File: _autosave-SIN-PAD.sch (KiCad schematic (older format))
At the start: 12 parts

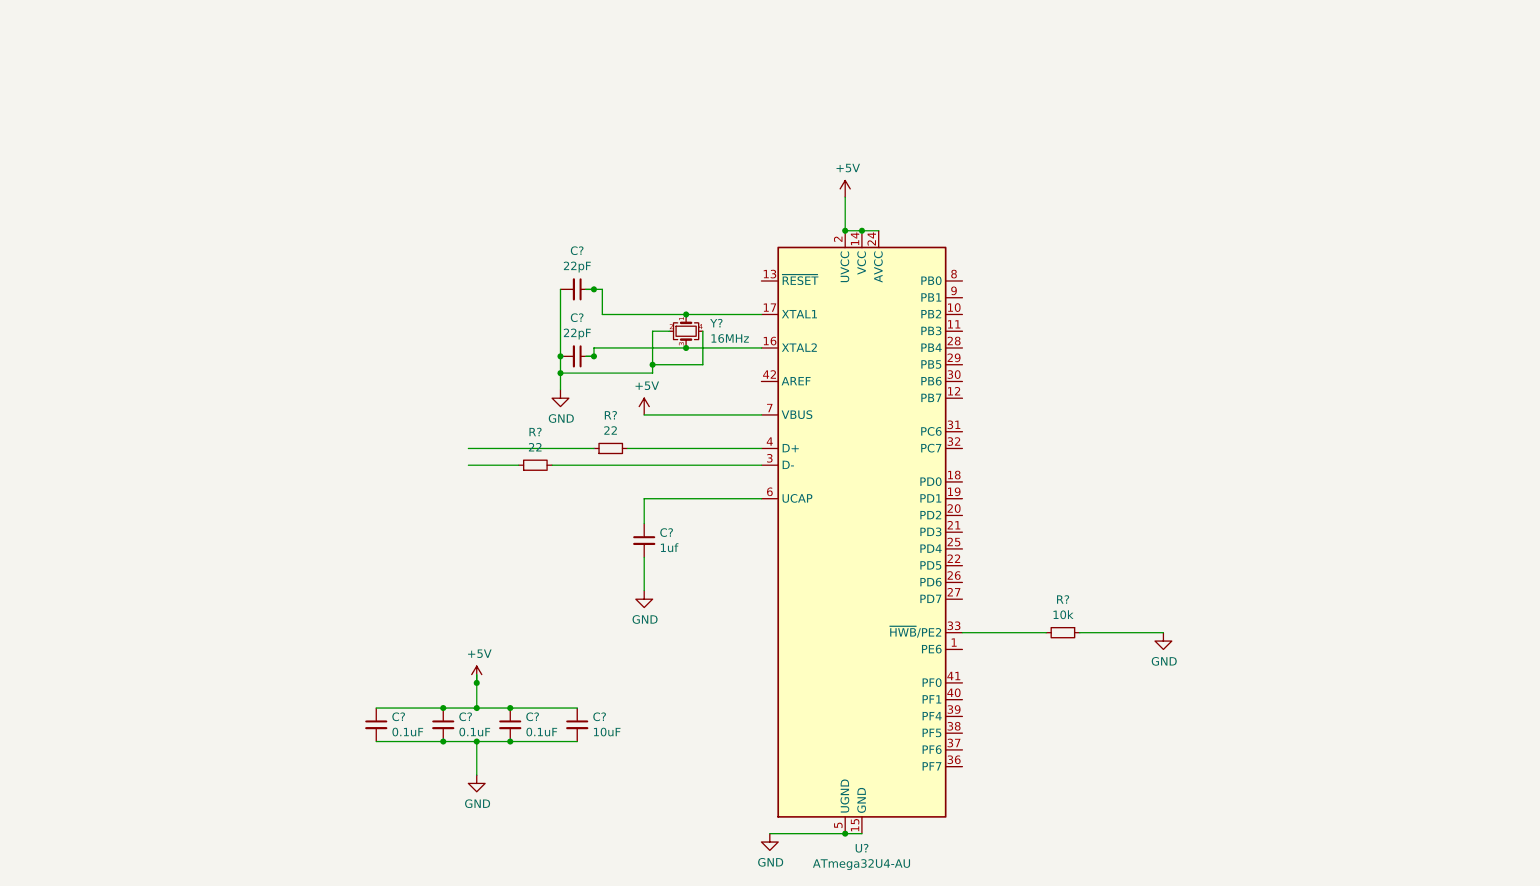
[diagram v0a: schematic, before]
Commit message: Kytkimet lätkitty tiskiin
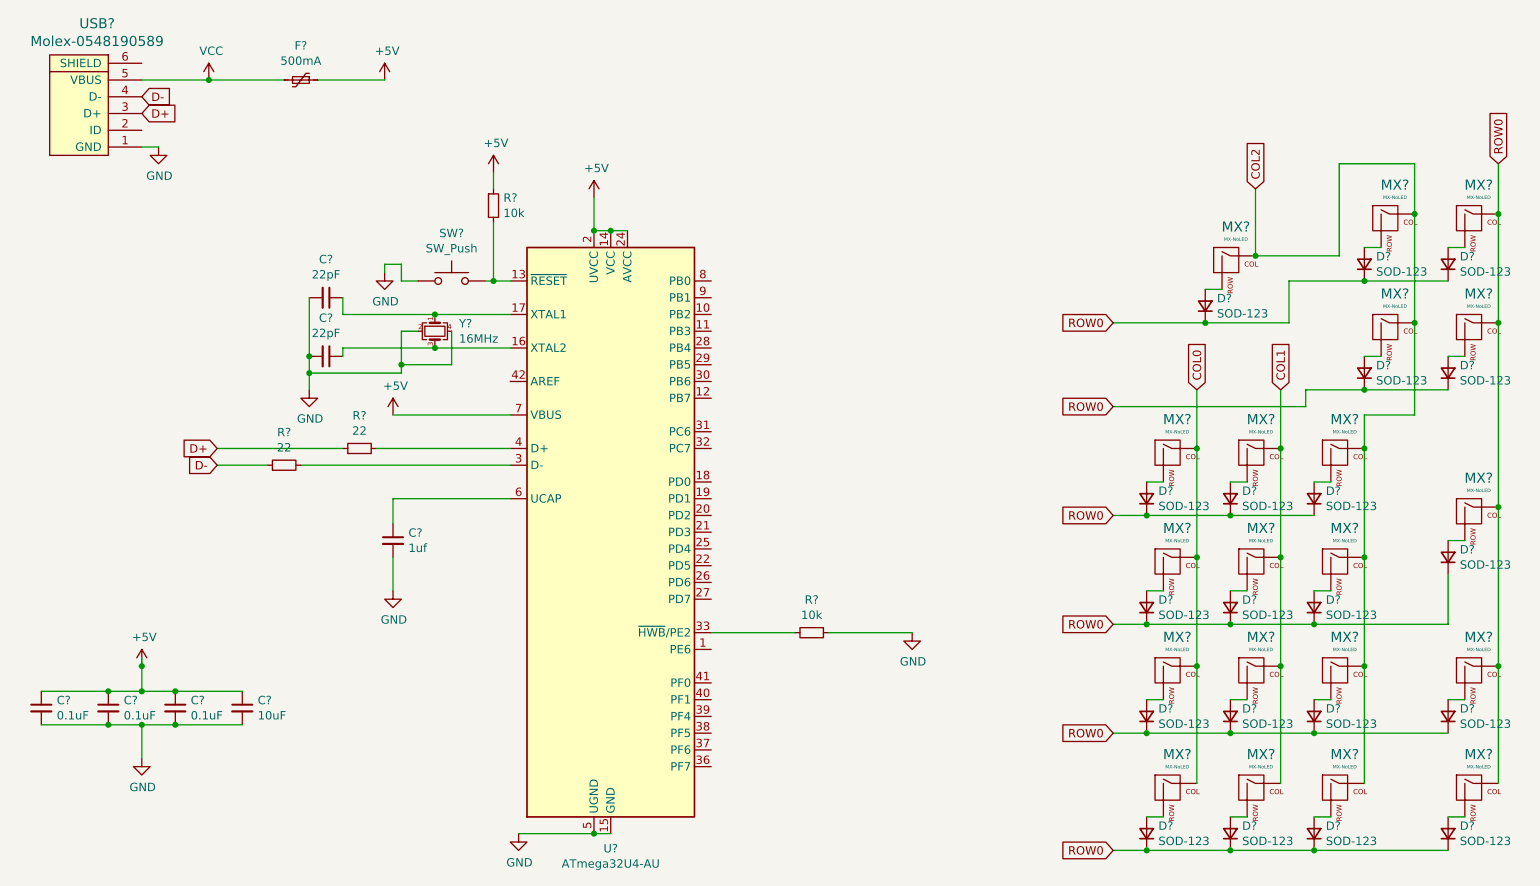
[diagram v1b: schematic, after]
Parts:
- added D? (x20): SOD-123, symbol Device:D_Small
- added F?: 500mA, symbol Device:Polyfuse_Small
- added MX? (x20): MX-NoLED, symbol MX_Alps_Hybrid:MX-NoLED
- added R?: 10k, symbol Device:R_Small
- added SW?: SW_Push, symbol Switch:SW_Push
- added USB?: Molex-0548190589, symbol random-keyboard-parts:Molex-0548190589
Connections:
- net labels added: COL0, COL1, COL2, D+, D-, ROW0, VCC
- wire segments 44 -> 123
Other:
- moved on the sheet: C?, R?, U?, Y?
